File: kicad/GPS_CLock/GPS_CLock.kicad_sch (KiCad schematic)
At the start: 45 parts, among them J101 DEBUG, SW101 BOOT_JMP, SW102 BTN_UP, SW103 BTN_DWN, SW104 RUN, U101 W25Q16JVUXIQ, U102 VEML7700-TR, U103 RP2040

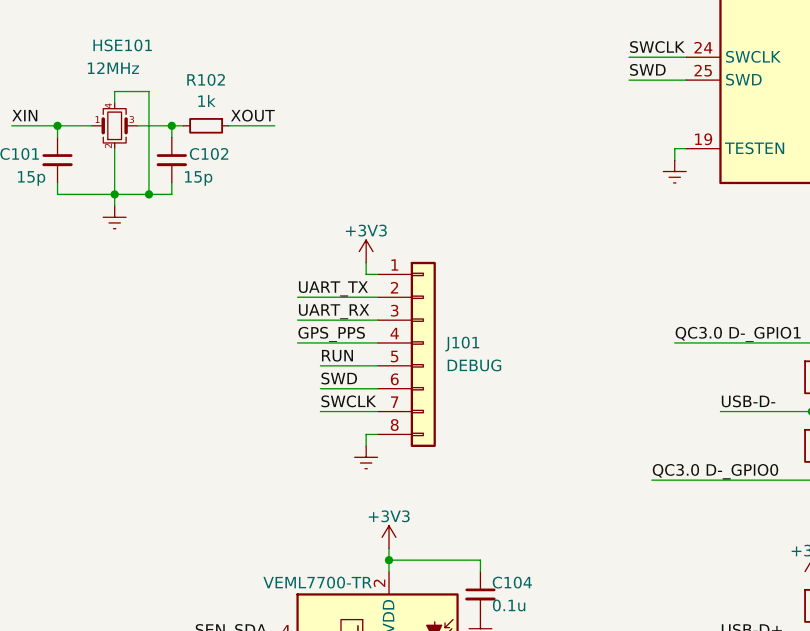
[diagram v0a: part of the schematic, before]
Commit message: update pcb
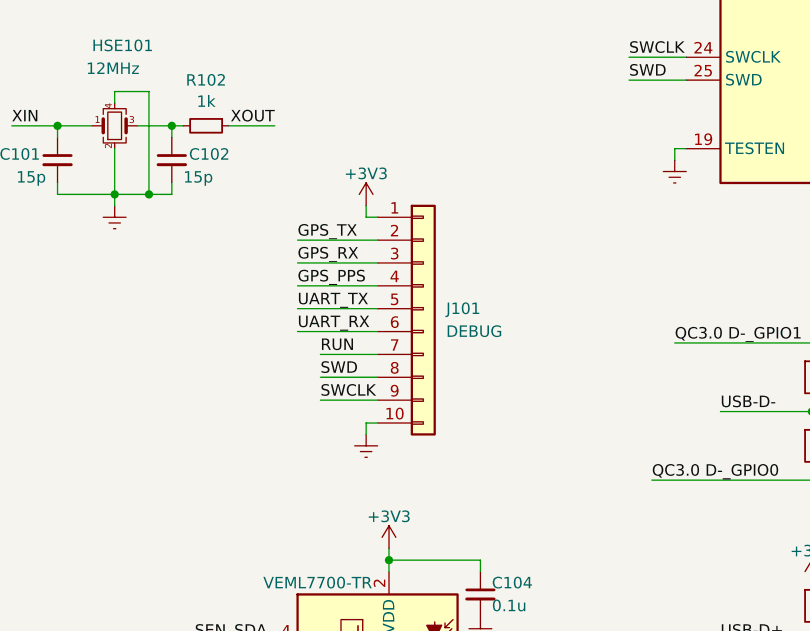
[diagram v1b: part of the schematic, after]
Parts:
- J101: footprint Connector_PinHeader_1.27mm:PinHeader_1x08_P1.27mm_Vertical -> Connector_PinHeader_2.54mm:PinHeader_1x10_P2.54mm_Vertical; symbol Connector_Generic:Conn_01x08 -> Connector_Generic:Conn_01x10
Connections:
- net Earth: now also J101.10 (Pin_10); no longer J101.8 (Pin_8)
- net GPS_RX: now also J101.3 (Pin_3)
- net GPS_TX: now also J101.2 (Pin_2)
- net RUN: now also J101.7 (Pin_7); no longer J101.5 (Pin_5)
- net SWCLK: now also J101.9 (Pin_9); no longer J101.7 (Pin_7)
- net SWD: now also J101.8 (Pin_8); no longer J101.6 (Pin_6)
- net UART_RX: now also J101.6 (Pin_6); no longer J101.3 (Pin_3)
- net UART_TX: now also J101.5 (Pin_5); no longer J101.2 (Pin_2)
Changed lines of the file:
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@@
     (stroke (width 0) (type default) (color 0 0 0 0))
   )
-  (wire (pts (xy 69.85 138.43) (xy 78.74 138.43))
+  (wire (pts (xy 69.85 139.7) (xy 78.74 139.7))
     (stroke (width 0) (type default) (color 0 0 0 0))
   )
@@
     (stroke (width 0) (type default) (color 0 0 0 0))
   )
+  (wire (pts (xy 69.85 132.08) (xy 78.74 132.08))
+    (stroke (width 0) (type default) (color 0 0 0 0))
+  )
   (wire (pts (xy 118.11 27.94) (xy 118.11 29.21))
     (stroke (width 0) (type default) (color 0 0 0 0))
   )
-  (wire (pts (xy 72.39 143.51) (xy 78.74 143.51))
+  (wire (pts (xy 72.39 142.24) (xy 78.74 142.24))
     (stroke (width 0) (type default) (color 0 0 0 0))
   )
@@
     (stroke (width 0) (type default) (color 0 0 0 0))
   )
-  (wire (pts (xy 77.47 132.08) (xy 77.47 133.35))
+  (wire (pts (xy 77.47 125.73) (xy 77.47 127))
     (stroke (width 0) (type default) (color 0 0 0 0))
   )
@@
     (stroke (width 0) (type default) (color 0 0 0 0))
   )
-  (wire (pts (xy 77.47 152.4) (xy 77.47 151.13))
+  (wire (pts (xy 77.47 151.13) (xy 77.47 149.86))
     (stroke (width 0) (type default) (color 0 0 0 0))
   )
@@
     (stroke (width 0) (type default) (color 0 0 0 0))
   )
-  (wire (pts (xy 69.85 135.89) (xy 78.74 135.89))
+  (wire (pts (xy 69.85 137.16) (xy 78.74 137.16))
     (stroke (width 0) (type default) (color 0 0 0 0))
   )
@@
     (stroke (width 0) (type default) (color 0 0 0 0))
   )
-  (wire (pts (xy 77.47 133.35) (xy 78.74 133.35))
+  (wire (pts (xy 77.47 127) (xy 78.74 127))
     (stroke (width 0) (type default) (color 0 0 0 0))
   )
@@
     (stroke (width 0) (type default) (color 0 0 0 0))
   )
-  (wire (pts (xy 72.39 148.59) (xy 78.74 148.59))
+  (wire (pts (xy 72.39 147.32) (xy 78.74 147.32))
     (stroke (width 0) (type default) (color 0 0 0 0))
   )
@@
     (stroke (width 0) (type default) (color 0 0 0 0))
   )
+  (wire (pts (xy 69.85 129.54) (xy 78.74 129.54))
+    (stroke (width 0) (type default) (color 0 0 0 0))
+  )
   (wire (pts (xy 205.74 27.94) (xy 214.63 27.94))
     (stroke (width 0) (type default) (color 0 0 0 0))
@@
     (stroke (width 0) (type default) (color 0 0 0 0))
   )
-  (wire (pts (xy 72.39 146.05) (xy 78.74 146.05))
+  (wire (pts (xy 72.39 144.78) (xy 78.74 144.78))
     (stroke (width 0) (type default) (color 0 0 0 0))
   )
@@
     (stroke (width 0) (type default) (color 0 0 0 0))
   )
-  (wire (pts (xy 78.74 140.97) (xy 69.85 140.97))
+  (wire (pts (xy 78.74 134.62) (xy 69.85 134.62))
     (stroke (width 0) (type default) (color 0 0 0 0))
   )
@@
     (stroke (width 0) (type default) (color 0 0 0 0))
   )
-  (wire (pts (xy 77.47 151.13) (xy 78.74 151.13))
+  (wire (pts (xy 77.47 149.86) (xy 78.74 149.86))
     (stroke (width 0) (type default) (color 0 0 0 0))
   )
@@
     (effects (font (size 1.27 1.27)) (justify right bottom))
   )
-  (label "RUN" (at 72.39 143.51 0)
+  (label "RUN" (at 72.39 142.24 0)
     (effects (font (size 1.27 1.27)) (justify left bottom))
   )
@@
     (effects (font (size 1.27 1.27)) (justify left bottom))
   )
-  (label "UART_TX" (at 69.85 135.89 0)
+  (label "UART_TX" (at 69.85 137.16 0)
     (effects (font (size 1.27 1.27)) (justify left bottom))
   )
@@
     (effects (font (size 1.27 1.27)) (justify right bottom))
   )
-  (label "GPS_PPS" (at 69.85 140.97 0)
+  (label "GPS_PPS" (at 69.85 134.62 0)
     (effects (font (size 1.27 1.27)) (justify left bottom))
   )
@@
     (effects (font (size 1.27 1.27)) (justify left bottom))
   )
-  (label "UART_RX" (at 69.85 138.43 0)
+  (label "UART_RX" (at 69.85 139.7 0)
     (effects (font (size 1.27 1.27)) (justify left bottom))
   )
@@
     (effects (font (size 1.27 1.27)) (justify left bottom))
   )
+  (label "GPS_TX" (at 69.85 129.54 0)
+    (effects (font (size 1.27 1.27)) (justify left bottom))
+  )
   (label "DISP_CLK" (at 177.8 68.58 180)
     (effects (font (size 1.27 1.27)) (justify right bottom))
@@
     (effects (font (size 1.27 1.27)) (justify left bottom))
   )
-  (label "SWCLK" (at 72.39 148.59 0)
+  (label "SWCLK" (at 72.39 147.32 0)
     (effects (font (size 1.27 1.27)) (justify left bottom))
   )
@@
     (effects (font (size 1.27 1.27)) (justify right bottom))
   )
+  (label "GPS_RX" (at 69.85 132.08 0)
+    (effects (font (size 1.27 1.27)) (justify left bottom))
+  )
   (label "BC_INT" (at 229.87 101.6 0)
     (effects (font (size 1.27 1.27)) (justify left bottom))
@@
     (effects (font (size 1.27 1.27)) (justify left bottom))
   )
-  (label "SWD" (at 72.39 146.05 0)
+  (label "SWD" (at 72.39 144.78 0)
     (effects (font (size 1.27 1.27)) (justify left bottom))
   )
@@
     (pin "2")
   )
-  (symbol (lib_id "power:Earth") (at 77.47 152.4 0) (unit 1)
+  (symbol (lib_id "power:Earth") (at 77.47 151.13 0) (unit 1)
     (in_bom yes) (on_board yes) (fields_autoplaced)
-    (property "Reference" "#PWR0107" (id 0) (at 77.47 158.75 0)
+    (property "Reference" "#PWR0107" (id 0) (at 77.47 157.48 0)
       (effects (font (size 1.27 1.27)) hide)
     )
-    (property "Value" "Earth" (id 1) (at 77.47 156.21 0)
+    (property "Value" "Earth" (id 1) (at 77.47 154.94 0)
       (effects (font (size 1.27 1.27)) hide)
     )
-    (property "Footprint" "" (id 2) (at 77.47 152.4 0)
+    (property "Footprint" "" (id 2) (at 77.47 151.13 0)
       (effects (font (size 1.27 1.27)) hide)
     )
-    (property "Datasheet" "~" (id 3) (at 77.47 152.4 0)
+    (property "Datasheet" "~" (id 3) (at 77.47 151.13 0)
       (effects (font (size 1.27 1.27)) hide)
     )
@@
     (pin "4")
   )
-  (symbol (lib_id "power:+3V3") (at 77.47 132.08 0) (unit 1)
+  (symbol (lib_id "power:+3V3") (at 77.47 125.73 0) (unit 1)
     (in_bom yes) (on_board yes)
-    (property "Reference" "#PWR0113" (id 0) (at 77.47 135.89 0)
+    (property "Reference" "#PWR0113" (id 0) (at 77.47 129.54 0)
       (effects (font (size 1.27 1.27)) hide)
     )
-    (property "Value" "+3V3" (id 1) (at 77.47 128.524 0))
-    (property "Footprint" "" (id 2) (at 77.47 132.08 0)
+    (property "Value" "+3V3" (id 1) (at 77.47 122.174 0))
+    (property "Footprint" "" (id 2) (at 77.47 125.73 0)
       (effects (font (size 1.27 1.27)) hide)
     )
-    (property "Datasheet" "" (id 3) (at 77.47 132.08 0)
+    (property "Datasheet" "" (id 3) (at 77.47 125.73 0)
       (effects (font (size 1.27 1.27)) hide)
     )
@@
     (pin "1")
   )
-  (symbol (lib_id "Connector_Generic:Conn_01x08") (at 83.82 140.97 0) (unit 1)
+  (symbol (lib_id "Connector_Generic:Conn_01x10") (at 83.82 137.16 0) (unit 1)
     (in_bom yes) (on_board yes) (fields_autoplaced)
-    (property "Reference" "J101" (id 0) (at 86.36 140.9699 0)
+    (property "Reference" "J101" (id 0) (at 86.36 137.1599 0)
       (effects (font (size 1.27 1.27)) (justify left))
     )
-    (property "Value" "DEBUG" (id 1) (at 86.36 143.5099 0)
+    (property "Value" "DEBUG" (id 1) (at 86.36 139.6999 0)
       (effects (font (size 1.27 1.27)) (justify left))
     )
-    (property "Footprint" "Connector_PinHeader_1.27mm:PinHeader_1x08_P1.27mm_Vertical" (id 2) (at 83.82 140.97 0)
+    (property "Footprint" "Connector_PinHeader_2.54mm:PinHeader_1x10_P2.54mm_Vertical" (id 2) (at 83.82 137.16 0)
       (effects (font (size 1.27 1.27)) hide)
     )
-    (property "Datasheet" "~" (id 3) (at 83.82 140.97 0)
+    (property "Datasheet" "~" (id 3) (at 83.82 137.16 0)
       (effects (font (size 1.27 1.27)) hide)
     )
     (pin "1")
+    (pin "10")
     (pin "2")
     (pin "3")
@@
     (pin "7")
     (pin "8")
+    (pin "9")
   )
   (symbol (lib_id "power:Earth") (at 22.86 78.74 0) (mirror y) (unit 1)
@@
     )
     (path "/d863043c-a8bd-4fef-b2a6-bef897c69d76"
-      (reference "J101") (unit 1) (value "DEBUG") (footprint "Connector_PinHeader_1.27mm:PinHeader_1x08_P1.27mm_Vertical")
+      (reference "J101") (unit 1) (value "DEBUG") (footprint "Connector_PinHeader_2.54mm:PinHeader_1x10_P2.54mm_Vertical")
     )
     (path "/1f693c02-7734-4d07-85c5-22483e243ef7/274b11b0-edb1-49fd-889c-a6f6718d1342"
@@
       (reference "SW104") (unit 1) (value "RUN") (footprint "clock:SW_SPST_EVQP2")
     )
+    (path "/1f693c02-7734-4d07-85c5-22483e243ef7/ce05c308-58db-43e5-9df3-a5f047177185"
+      (reference "TP201") (unit 1) (value "VBUS") (footprint "TestPoint:TestPoint_Bridge_Pitch2.0mm_Drill0.7mm")
+    )
+    (path "/1f693c02-7734-4d07-85c5-22483e243ef7/e591a947-dda1-46c3-9519-a81a413319db"
+      (reference "TP202") (unit 1) (value "2V5_TOP") (footprint "TestPoint:TestPoint_Bridge_Pitch2.0mm_Drill0.7mm")
+    )
+    (path "/1f693c02-7734-4d07-85c5-22483e243ef7/0667ef4c-0946-4dee-8919-a8a913a74a94"
+      (reference "TP203") (unit 1) (value "2.5V_BOT") (footprint "TestPoint:TestPoint_Bridge_Pitch2.0mm_Drill0.7mm")
+    )
+    (path "/1f693c02-7734-4d07-85c5-22483e243ef7/e517c2d8-778e-4d4e-9c74-8461bb379564"
+      (reference "TP204") (unit 1) (value "3V3") (footprint "TestPoint:TestPoint_Bridge_Pitch2.0mm_Drill0.7mm")
+    )
     (path "/b616feb9-0dfe-4528-bc37-d0e6cae1b2c9"
